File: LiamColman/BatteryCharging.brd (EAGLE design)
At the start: 34.5 x 47.9 mm, 3 parts, among them X1 MAB5SV, X2 MAB5SV

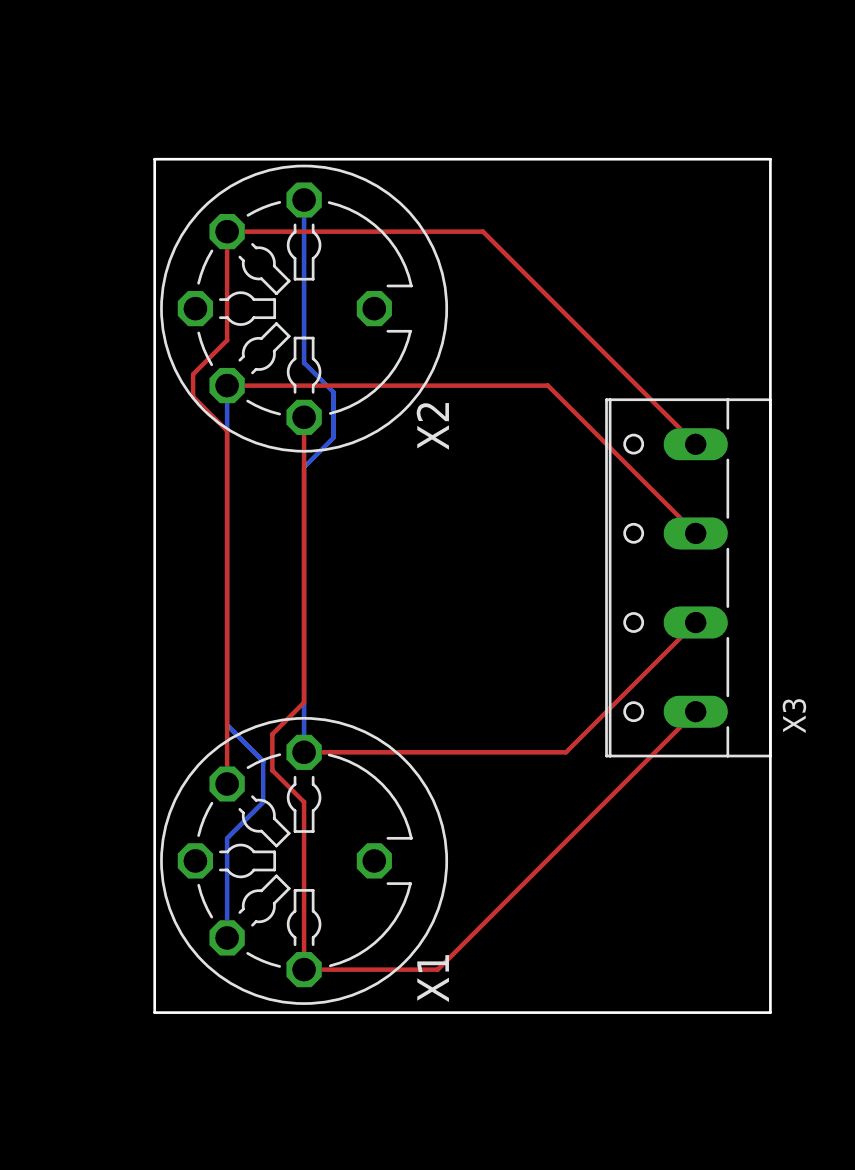
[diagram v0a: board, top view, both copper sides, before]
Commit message: Updated Battery PCB files
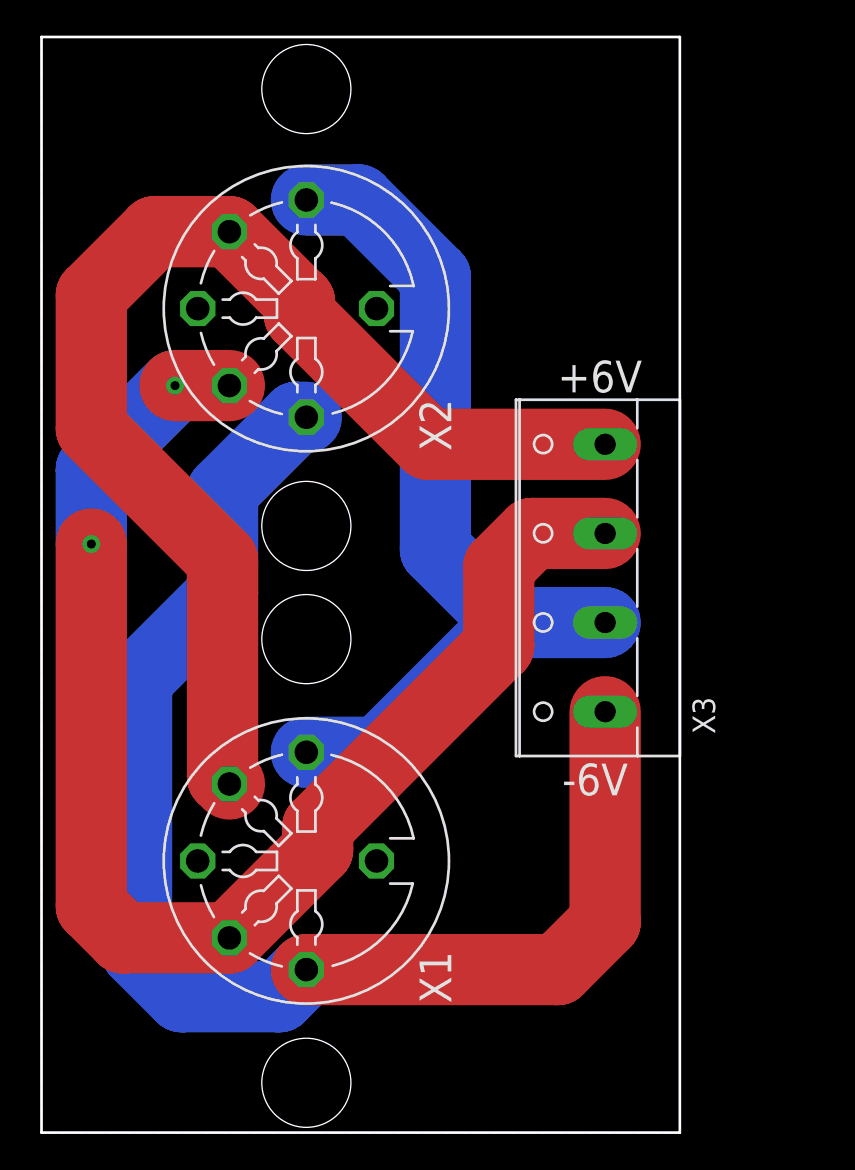
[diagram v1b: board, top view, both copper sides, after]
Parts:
- moved X3 5.08 mm to (45.3, 41.3)
- moved X1 0.13 mm to (29.8, 25.4)
- moved X2 0.13 mm to (29.8, 56.4)
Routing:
- net -6V: track 60.4 -> 75.1 mm
- net +0V: track 62.4 -> 76.5 mm, vias 0 -> 2
- net -0V: track 57.3 -> 49.9 mm
- net +6V: track 63.8 -> 66.3 mm
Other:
- board size 34.5 x 47.9 mm -> 35.8 x 61.5 mm
- board text added: "+6V"
- board text added: "-6V"

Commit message: Updated PCB design & Gerber files
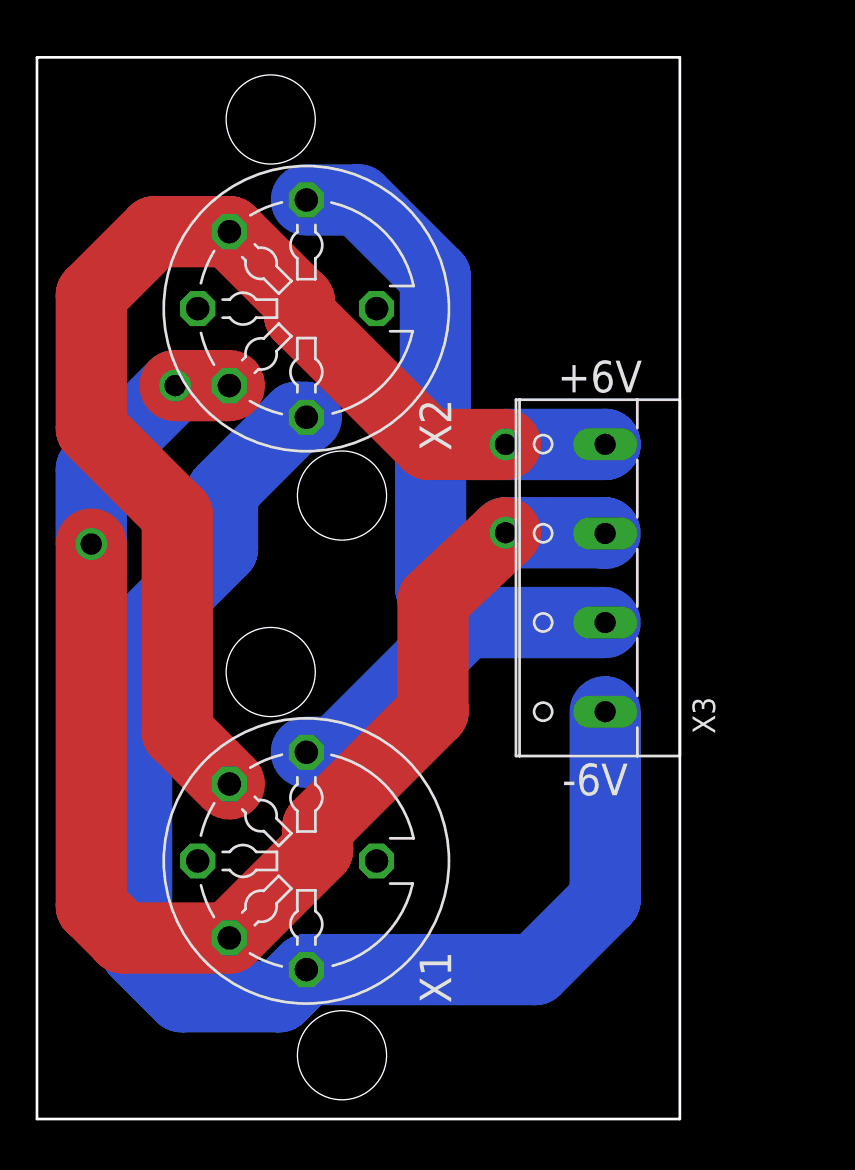
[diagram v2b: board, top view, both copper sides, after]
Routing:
- net +0V: track 76.5 -> 77.5 mm, vias 2 -> 3
- net -0V: track 49.9 -> 49.1 mm
- net -6V: track 75.1 -> 74.4 mm
- net +6V: vias 0 -> 1
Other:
- board size 35.8 x 61.5 mm -> 36.1 x 59.6 mm
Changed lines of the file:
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@@
 <layer number="42" name="bRestrict" color="1" fill="10" visible="yes" active="yes"/>
 <layer number="43" name="vRestrict" color="2" fill="10" visible="yes" active="yes"/>
-<layer number="44" name="Drills" color="7" fill="1" visible="no" active="yes"/>
+<layer number="44" name="Drills" color="7" fill="1" visible="yes" active="yes"/>
 <layer number="45" name="Holes" color="7" fill="1" visible="yes" active="yes"/>
 <layer number="46" name="Milling" color="3" fill="1" visible="no" active="yes"/>
@@
 <board>
 <plain>
-<wire x1="14.986" y1="10.16" x2="14.986" y2="71.628" width="0.15" layer="20"/>
-<wire x1="14.986" y1="71.628" x2="50.8" y2="71.628" width="0.15" layer="20"/>
-<wire x1="50.8" y1="71.628" x2="50.8" y2="10.16" width="0.15" layer="20"/>
-<wire x1="50.8" y1="10.16" x2="14.986" y2="10.16" width="0.15" layer="20"/>
+<wire x1="14.732" y1="10.922" x2="14.732" y2="70.485" width="0.15" layer="20"/>
+<wire x1="14.732" y1="70.485" x2="50.8" y2="70.485" width="0.15" layer="20"/>
+<wire x1="50.8" y1="70.485" x2="50.8" y2="10.922" width="0.15" layer="20"/>
+<wire x1="50.8" y1="10.922" x2="14.732" y2="10.922" width="0.15" layer="20"/>
 <text x="43.942" y="51.689" size="1.778" layer="21">+6V</text>
 <text x="44.196" y="29.083" size="1.778" layer="21">-6V</text>
-<hole x="29.845" y="12.954" drill="5"/>
-<hole x="29.845" y="37.846" drill="5"/>
-<hole x="29.845" y="44.196" drill="5"/>
-<hole x="29.845" y="68.707" drill="5"/>
-<dimension x1="14.986" y1="71.628" x2="50.8" y2="71.628" x3="32.893" y3="74.93" textsize="1.778" layer="1" dtype="vertical"/>
-<dimension x1="14.986" y1="10.16" x2="14.986" y2="71.628" x3="8.89" y3="40.894" textsize="1.778" layer="1" dtype="vertical"/>
+<hole x="31.845" y="14.5" drill="5"/>
+<hole x="27.845" y="36" drill="5"/>
+<hole x="31.845" y="45.9" drill="5"/>
+<hole x="27.845" y="67" drill="5"/>
 </plain>
 <attributes>
@@
 <contactref element="X2" pad="3"/>
 <contactref element="X3" pad="2"/>
-<wire x1="29.845" y1="31.496" x2="33.909" y2="31.496" width="4" layer="16"/>
-<wire x1="46.609" y1="38.775" x2="41.188" y2="38.775" width="4" layer="16"/>
-<wire x1="33.909" y1="31.496" x2="41.188" y2="38.775" width="4" layer="16"/>
+<wire x1="29.845" y1="31.496" x2="31.496" y2="31.496" width="4" layer="16"/>
+<wire x1="46.609" y1="38.775" x2="38.775" y2="38.775" width="4" layer="16"/>
+<wire x1="31.496" y1="31.496" x2="38.775" y2="38.775" width="4" layer="16"/>
 <wire x1="29.845" y1="62.484" x2="32.766" y2="62.484" width="4" layer="16"/>
-<wire x1="37.084" y1="58.166" x2="32.766" y2="62.484" width="4" layer="16"/>
-<wire x1="41.188" y1="38.775" x2="37.084" y2="42.879" width="4" layer="16"/>
-<wire x1="37.084" y1="42.879" x2="37.084" y2="58.166" width="4" layer="16"/>
+<wire x1="32.766" y1="62.484" x2="37.084" y2="58.166" width="4" layer="16"/>
+<wire x1="37.084" y1="50.775225" x2="36.8178" y2="50.509025" width="4" layer="16"/>
+<wire x1="36.8178" y1="50.509025" x2="36.8178" y2="40.7322" width="4" layer="16"/>
+<wire x1="36.8178" y1="40.7322" x2="38.775" y2="38.775" width="4" layer="16"/>
+<wire x1="37.084" y1="58.166" x2="37.084" y2="50.775225" width="4" layer="16"/>
 </signal>
 <signal name="+6V">
@@
 <wire x1="21.336" y1="60.706" x2="17.78" y2="57.15" width="4" layer="1"/>
 <wire x1="17.78" y1="57.15" x2="17.78" y2="49.657" width="4" layer="1"/>
-<wire x1="17.78" y1="49.657" x2="25.1418" y2="42.2952" width="4" layer="1"/>
-<wire x1="25.1418" y1="30.1032" x2="25.527" y2="29.718" width="4" layer="1"/>
-<wire x1="25.1418" y1="42.2952" x2="25.1418" y2="30.1032" width="4" layer="1"/>
+<wire x1="17.78" y1="49.657" x2="22.6018" y2="44.8352" width="4" layer="1"/>
+<wire x1="22.6018" y1="32.6432" x2="25.527" y2="29.718" width="4" layer="1"/>
+<wire x1="22.6018" y1="44.8352" x2="22.6018" y2="32.6432" width="4" layer="1"/>
 <wire x1="25.527" y1="60.706" x2="29.464" y2="56.769" width="4" layer="1"/>
 <wire x1="29.464" y1="56.769" x2="29.464" y2="56.007" width="4" layer="1"/>
-<wire x1="29.464" y1="56.007" x2="36.696" y2="48.775" width="4" layer="1"/>
-<wire x1="36.696" y1="48.775" x2="46.609" y2="48.775" width="4" layer="1"/>
+<wire x1="36.703" y1="48.768" x2="41.021" y2="48.768" width="4" layer="1"/>
+<via x="41.021" y="48.768" extent="1-16" drill="1.2"/>
+<wire x1="41.021" y1="48.768" x2="46.602" y2="48.768" width="4" layer="16"/>
+<wire x1="46.602" y1="48.768" x2="46.609" y2="48.775" width="4" layer="16"/>
+<wire x1="29.464" y1="56.007" x2="36.703" y2="48.768" width="4" layer="1"/>
 </signal>
 <signal name="+0V">
@@
 <wire x1="25.527" y1="21.082" x2="30.48" y2="26.035" width="4" layer="1"/>
 <wire x1="30.48" y1="26.035" x2="30.48" y2="27.305" width="4" layer="1"/>
-<wire x1="40.64" y1="37.465" x2="40.64" y2="41.91" width="4" layer="1"/>
-<wire x1="40.64" y1="41.91" x2="42.505" y2="43.775" width="4" layer="1"/>
-<wire x1="42.505" y1="43.775" x2="46.609" y2="43.775" width="4" layer="1"/>
-<wire x1="30.48" y1="27.305" x2="40.64" y2="37.465" width="4" layer="1"/>
+<wire x1="30.48" y1="27.305" x2="36.957" y2="33.782" width="4" layer="1"/>
 <wire x1="17.78" y1="22.86" x2="17.78" y2="43.18" width="4" layer="1"/>
-<via x="17.78" y="43.18" extent="1-16" drill="0.508"/>
+<via x="17.78" y="43.18" extent="1-16" drill="1.2"/>
 <wire x1="17.78" y1="43.18" x2="17.78" y2="47.371" width="4" layer="16"/>
 <wire x1="17.78" y1="47.371" x2="22.479" y2="52.07" width="4" layer="16"/>
-<via x="22.479" y="52.07" extent="1-16" drill="0.508"/>
+<via x="22.479" y="52.07" extent="1-16" drill="1.2"/>
 <wire x1="22.479" y1="52.07" x2="25.527" y2="52.07" width="4" layer="1"/>
+<wire x1="36.957" y1="40.005" x2="41.021" y2="43.815" width="4" layer="1"/>
+<via x="41.021" y="43.815" extent="1-16" drill="1.2"/>
+<wire x1="41.021" y1="43.815" x2="46.569" y2="43.815" width="4" layer="16"/>
+<wire x1="46.569" y1="43.815" x2="46.609" y2="43.775" width="4" layer="16"/>
+<wire x1="36.957" y1="33.782" x2="36.957" y2="40.005" width="4" layer="1"/>
 </signal>
 <signal name="-6V">
@@
 <wire x1="29.845" y1="19.304" x2="28.321" y2="17.78" width="4" layer="16"/>
 <wire x1="28.321" y1="17.78" x2="22.86" y2="17.78" width="4" layer="16"/>
-<wire x1="29.845" y1="19.304" x2="43.942" y2="19.304" width="4" layer="1"/>
-<wire x1="43.942" y1="19.304" x2="46.609" y2="21.971" width="4" layer="1"/>
-<wire x1="46.609" y1="21.971" x2="46.609" y2="33.775" width="4" layer="1"/>
 <wire x1="22.86" y1="17.78" x2="20.32" y2="20.32" width="4" layer="16"/>
-<wire x1="25.1418" y1="40.3818" x2="25.1418" y2="46.14413125" width="4" layer="16"/>
-<wire x1="20.32" y1="20.32" x2="20.32" y2="35.56" width="4" layer="16"/>
-<wire x1="20.32" y1="35.56" x2="25.1418" y2="40.3818" width="4" layer="16"/>
+<wire x1="25.1418" y1="42.9218" x2="25.1418" y2="46.14413125" width="4" layer="16"/>
+<wire x1="20.32" y1="20.32" x2="20.32" y2="38.1" width="4" layer="16"/>
+<wire x1="20.32" y1="38.1" x2="25.1418" y2="42.9218" width="4" layer="16"/>
 <wire x1="25.1418" y1="46.14413125" x2="29.28966875" y2="50.292" width="4" layer="16"/>
 <wire x1="29.28966875" y1="50.292" x2="29.845" y2="50.292" width="4" layer="16"/>
+<wire x1="29.845" y1="19.304" x2="42.672" y2="19.304" width="4" layer="16"/>
+<wire x1="42.672" y1="19.304" x2="46.609" y2="23.241" width="4" layer="16"/>
+<wire x1="46.609" y1="23.241" x2="46.609" y2="33.775" width="4" layer="16"/>
 </signal>
 <signal name="GND">
@@
 <contactref element="X2" pad="2"/>
 <polygon width="0.254" layer="1" isolate="0.3048">
-<vertex x="14.986" y="71.628"/>
-<vertex x="50.8" y="71.628"/>
-<vertex x="50.8" y="10.16"/>
-<vertex x="14.986" y="10.16"/>
+<vertex x="14.732" y="70.485"/>
+<vertex x="50.8" y="70.485"/>
+<vertex x="50.8" y="10.922"/>
+<vertex x="14.732" y="10.922"/>
 </polygon>
 <polygon width="0.254" layer="16" isolate="0.3048">
-<vertex x="14.986" y="71.628"/>
-<vertex x="50.8" y="71.628"/>
-<vertex x="50.8" y="10.16"/>
-<vertex x="14.986" y="10.16"/>
+<vertex x="14.732" y="70.485"/>
+<vertex x="50.8" y="70.485"/>
+<vertex x="50.8" y="10.922"/>
+<vertex x="14.732" y="10.922"/>
 </polygon>
 <contactref element="X2" pad="PE"/>
